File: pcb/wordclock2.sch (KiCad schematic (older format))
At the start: 48 parts, among them J1 Jack-DC, J2 CONN_02X05, J3 Micro_SD_Card_Det, J4 USB_OTG, J5 CONN_01X03, J6 CONN_01X03, Q1 FDS6890A, SW1 SW_Push, SW2 SW_Push, SW3 SW_Push, SW4 SW_Push, U1 MAXIM_MAX44009, U2 Si7021, U3 TPS77833_SO8, U4 STM32L433CCT6, U5 ESP-12E, Y1 8MHz, Y2 32.768kHz

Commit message: progress
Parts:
- BT1: footprint (none) -> Connect:CR2032H
- J1: footprint (none) -> Connect:BARREL_JACK
- J4: footprint (none) -> Connect:USB_Micro-B
- U2: footprint (none) -> wordclockFB:Si7021-A20
- U5: footprint (none) -> ESP8266:ESP-12E_SMD

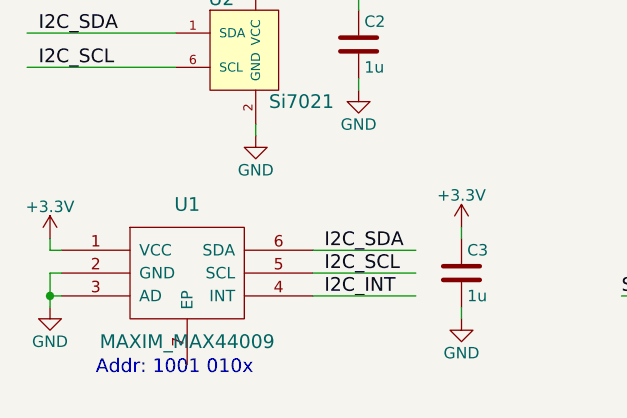
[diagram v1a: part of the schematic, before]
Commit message: progress
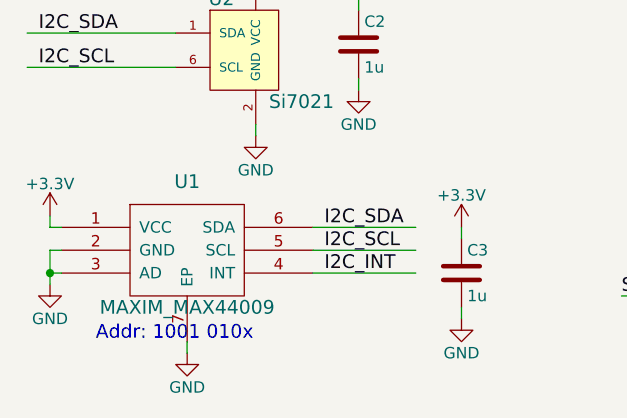
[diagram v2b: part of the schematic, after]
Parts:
- U1: footprint (none) -> wordclockFB:MAX44009
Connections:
- wire segments 201 -> 202
